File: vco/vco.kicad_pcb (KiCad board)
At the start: 2 copper layers, 66 x 99.1 mm, 63 parts, among them J1 Filtered Power, J13 Octave, J2 SQR, J3 TRI, J4 RMP, J5 1VO, J6 CV, J7 SNC, J8 PWM, J9 FM, U1 TL074, U2 TL072, U3 AS3340, U4 LM4040

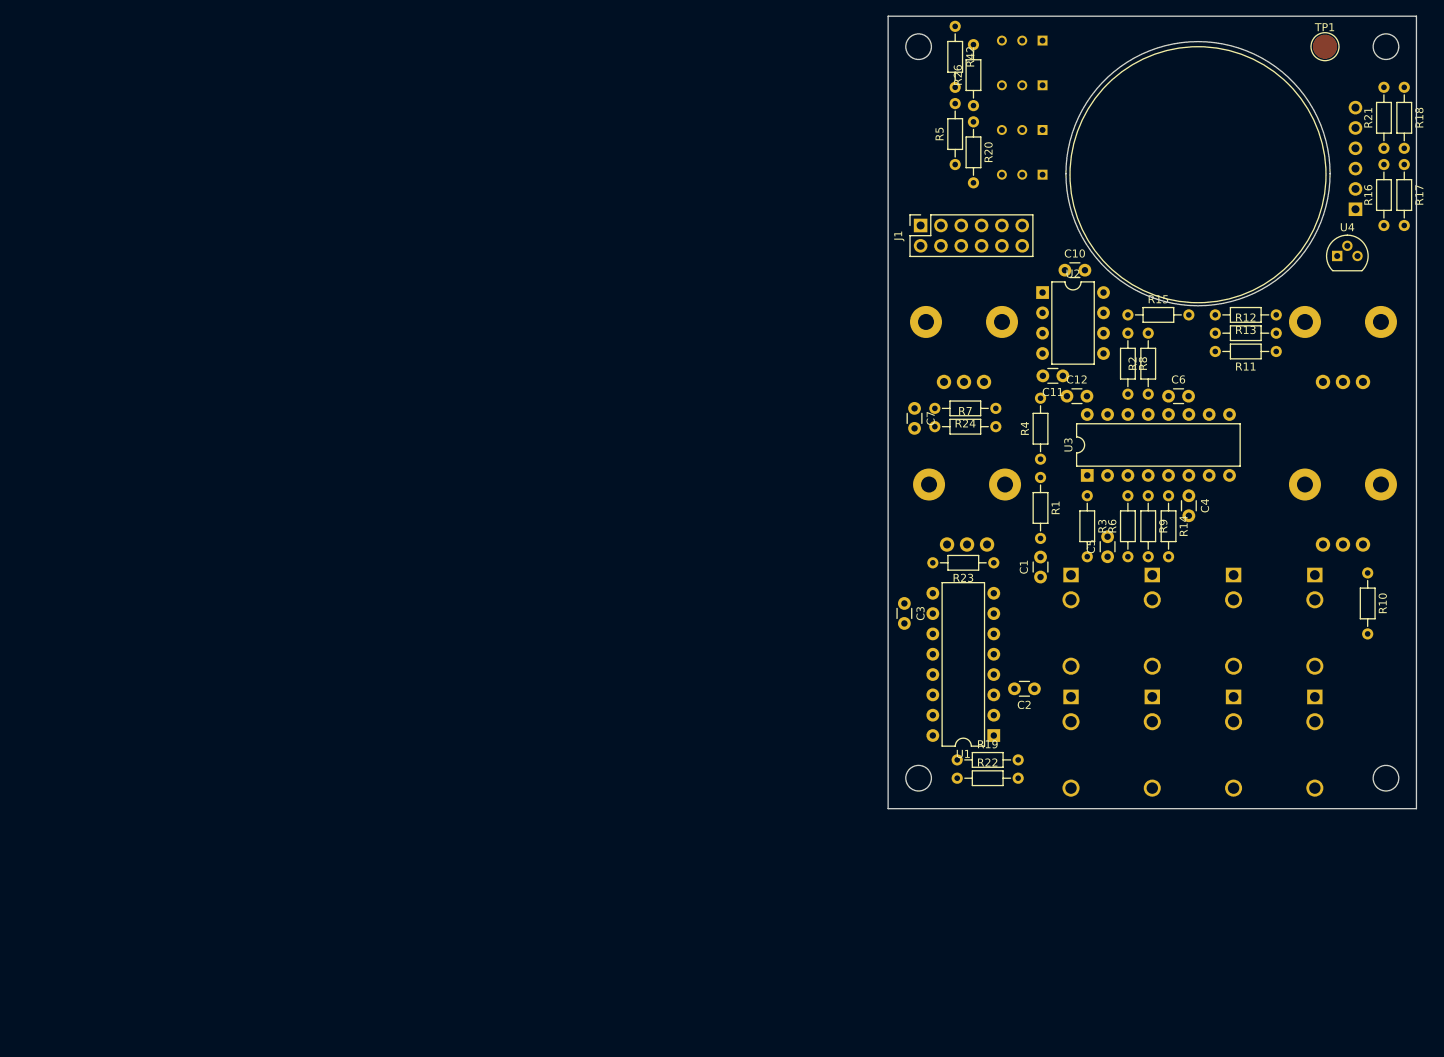
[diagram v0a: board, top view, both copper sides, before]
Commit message: Settled at larger pcb, think its going to work with components placed like this
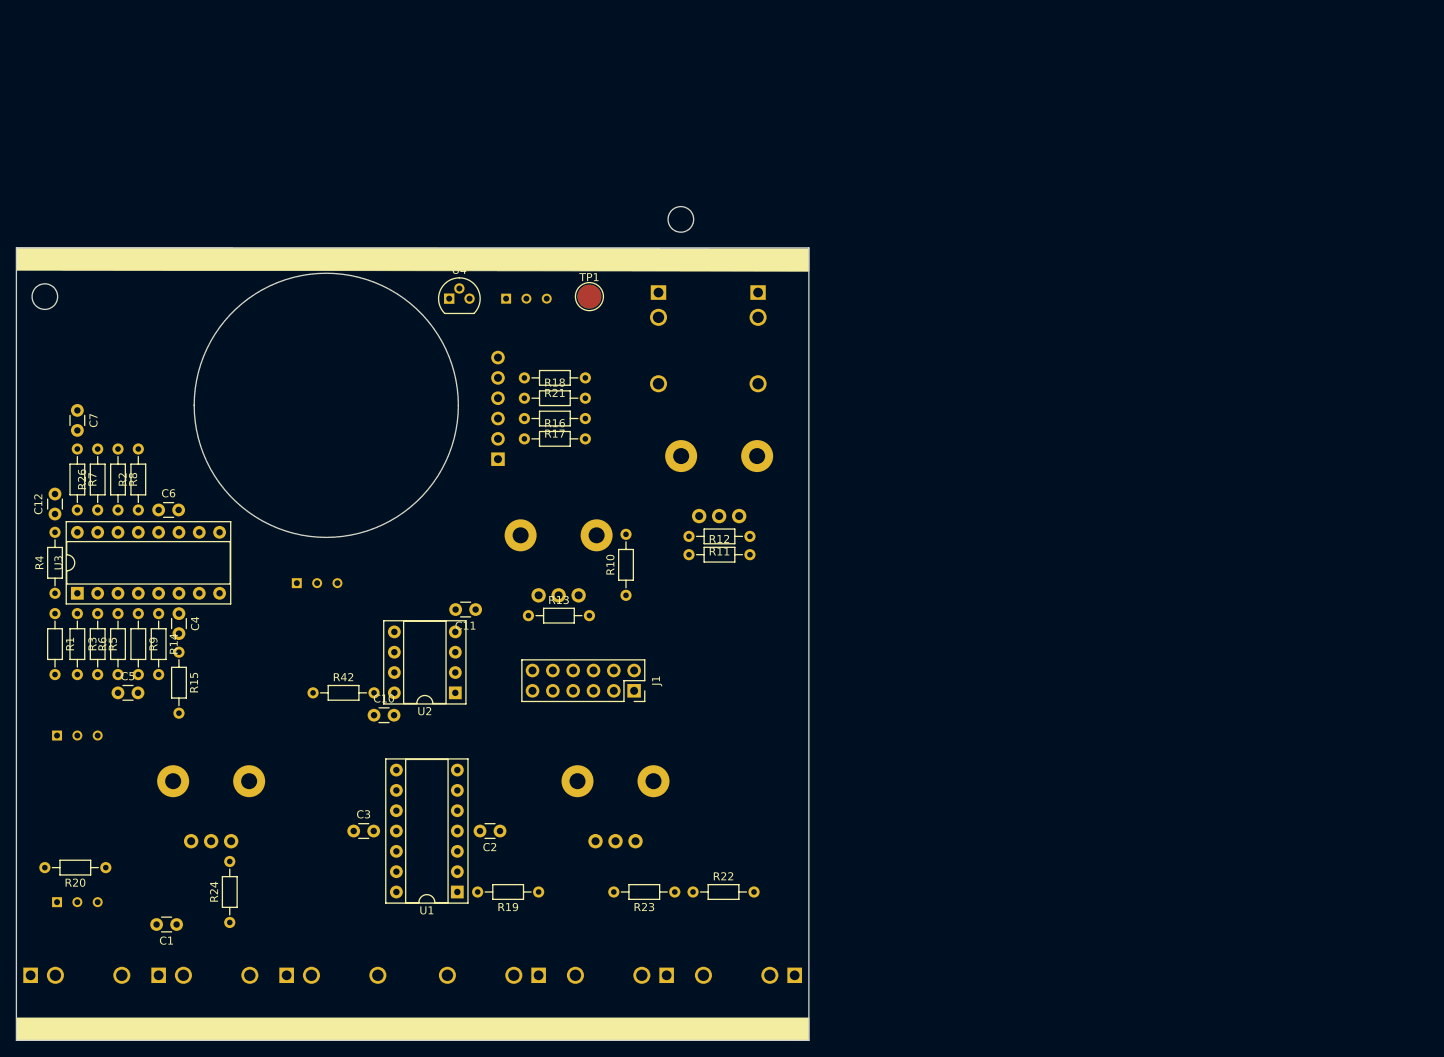
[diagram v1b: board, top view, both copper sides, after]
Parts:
- removed H2, H4: MountingHole, MountingHole:MountingHole_3.2mm_M3
- U1: footprint Package_DIP:DIP-16_W7.62mm -> Package_DIP:DIP-14_W7.62mm_Socket
- U2: footprint Package_DIP:DIP-8_W7.62mm -> Package_DIP:DIP-8_W7.62mm_Socket
- U3: footprint Package_DIP:DIP-16_W7.62mm -> Package_DIP:DIP-16_W7.62mm_Socket
- moved J6 164.3 mm to (83.3, 147.8), turned to 270 degrees
- moved RV5 149.1 mm to (89.2, 138.7), turned to 0 degrees
- moved R20 143.0 mm to (92.7, 134.4), turned to 180 degrees
- moved RV1 140.3 mm to (89.2, 117.9), turned to 0 degrees
- moved C12 127.3 mm to (86.4, 90.2), turned to 90 degrees
- moved C4 127.1 mm to (101.9, 102.6)
- moved R6 127.1 mm to (94.2, 110.2)
- moved R14 127.1 mm to (99.3, 102.6)
- moved R3 127.1 mm to (89.2, 102.6)
- moved R9 127.1 mm to (96.8, 102.6)
- moved U3 127.1 mm to (89.2, 100.1)
- moved R8 127.1 mm to (94.2, 82.0)
- moved R2 127.1 mm to (96.8, 89.7)
- moved C6 127.0 mm to (99.3, 89.7)
- moved R15 125.9 mm to (101.9, 107.4), turned to 270 degrees
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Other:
- board size 66 x 99.1 mm -> 99.1 x 99.1 mm
